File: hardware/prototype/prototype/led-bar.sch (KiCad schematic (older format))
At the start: 50 parts

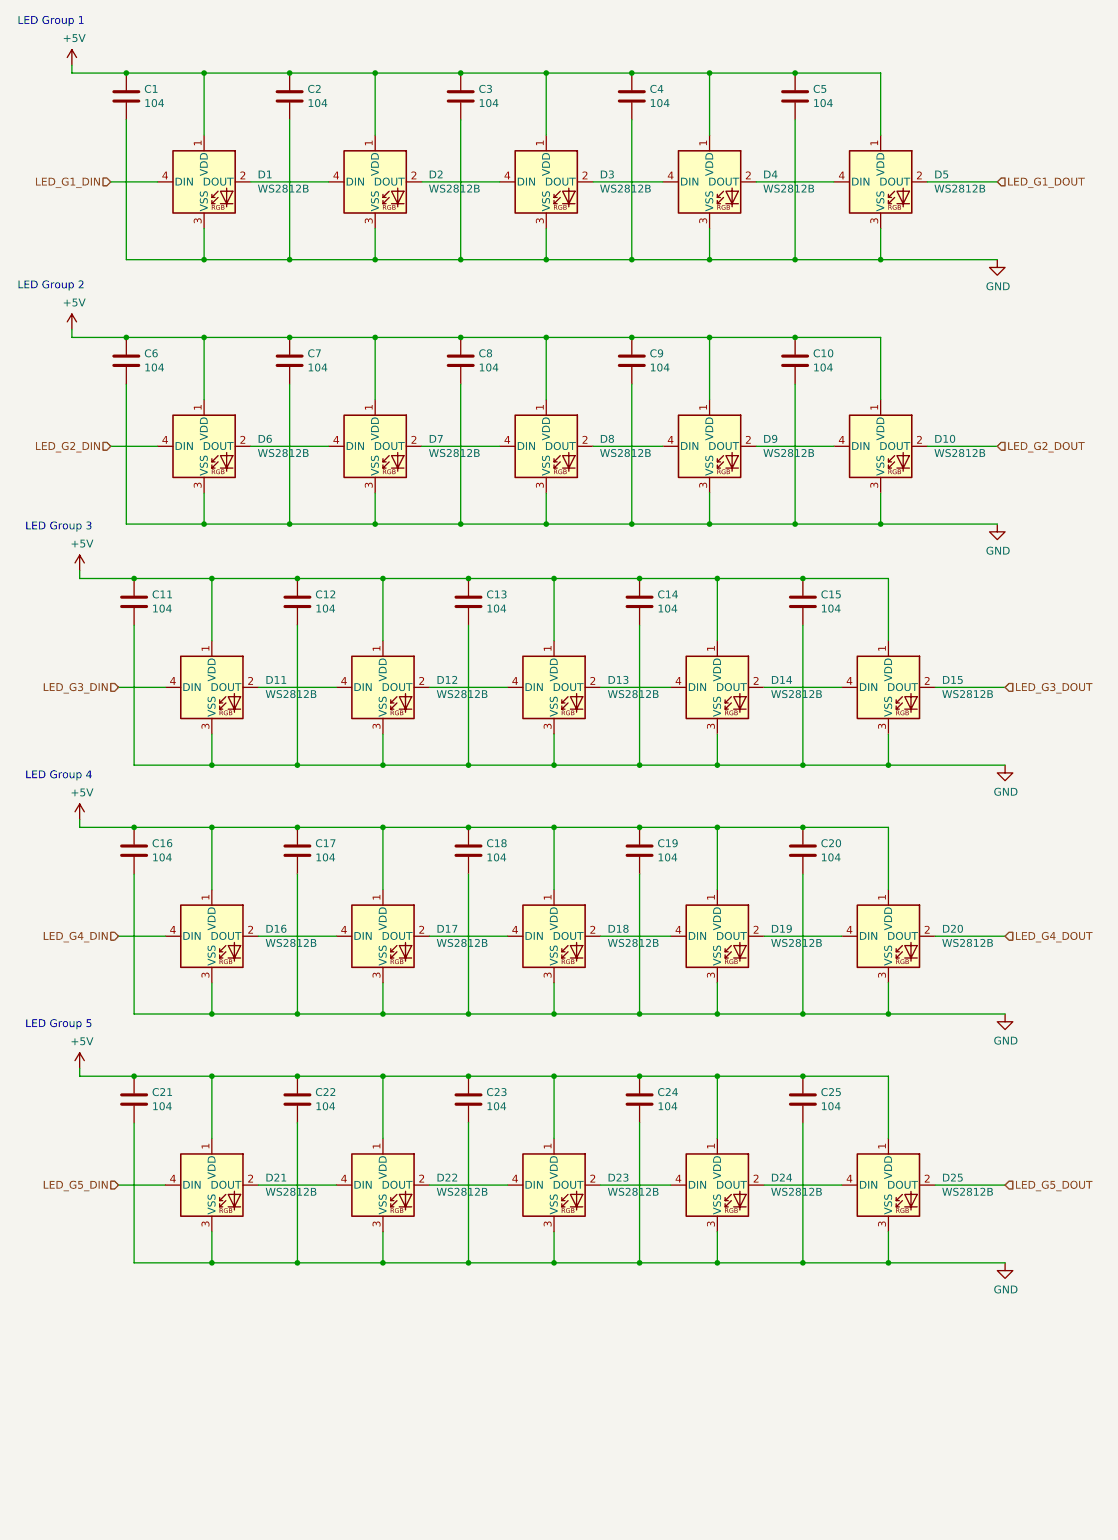
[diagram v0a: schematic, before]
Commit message: Update proto bar
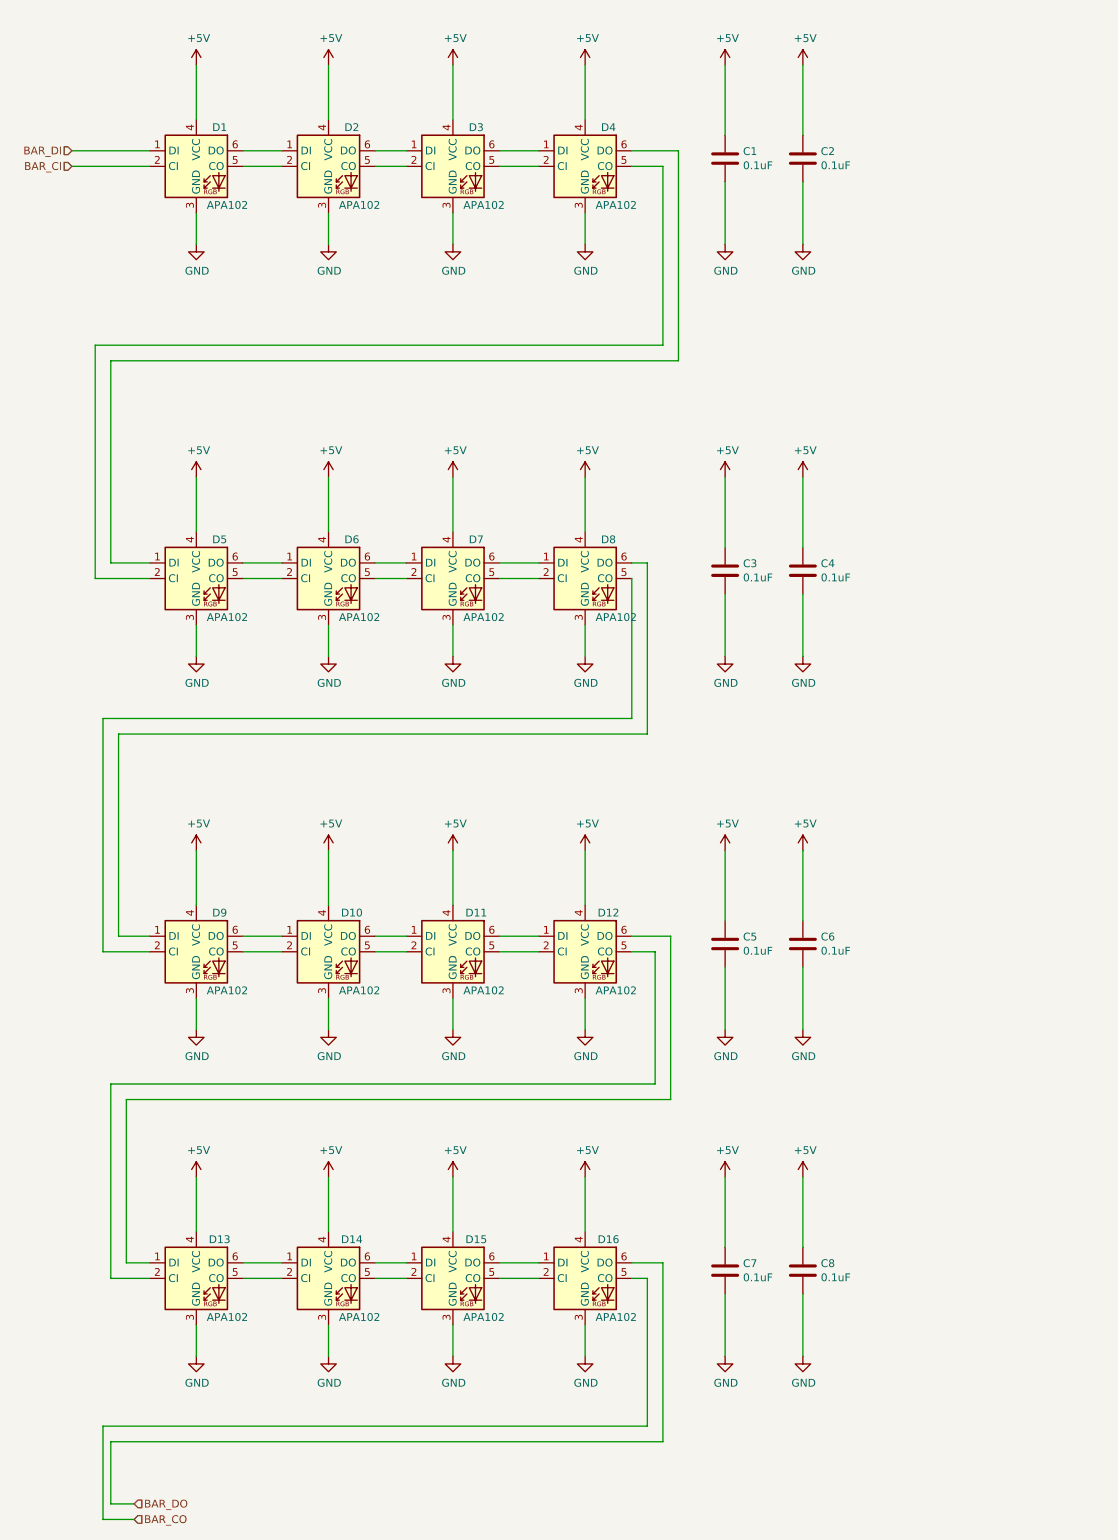
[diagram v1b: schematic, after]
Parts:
- removed C10, C11, C12, C13, C14, C15, C16, C17, C18, C19, C20, C21, C22, C23, C24, C25, C9: 104, Capacitor_SMD:C_0805_2012Metric, symbol Device:C
- removed D1, D10, D11, D12, D13, D14, D15, D16, D17, D18, D19, D2, D20, D21, D22, D23, D24, D25, D3, D4, D5, D6, D7, D8, D9: WS2812B, LED_SMD:LED_WS2812B_PLCC4_5.0x5.0mm_P3.2mm, symbol LED:WS2812B
- added D1, D10, D11, D12, D13, D14, D15, D16, D2, D3, D4, D5, D6, D7, D8, D9: APA102, LED_SMD:LED_RGB_5050-6, symbol LED:APA102
- C1, C2, C3, C4, C5, C6, C7, C8: value 104 -> 0.1uF; footprint Capacitor_SMD:C_0805_2012Metric -> Capacitor_SMD:C_0603_1608Metric
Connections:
- net +5V: now also D1.4 (VCC), D10.4 (VCC), D11.4 (VCC), D12.4 (VCC), D13.4 (VCC), D14.4 (VCC), D15.4 (VCC), D16.4 (VCC), D2.4 (VCC), D3.4 (VCC), D4.4 (VCC), D5.4 (VCC), D6.4 (VCC), D7.4 (VCC), D8.4 (VCC), D9.4 (VCC)
- net GND: now also D1.3 (GND), D10.3 (GND), D11.3 (GND), D12.3 (GND), D13.3 (GND), D14.3 (GND), D15.3 (GND), D16.3 (GND), D2.3 (GND), D3.3 (GND), D4.3 (GND), D5.3 (GND), D6.3 (GND), D7.3 (GND), D8.3 (GND), D9.3 (GND)
- new net: D1.5 (CO), D2.2 (CI)
- new net: D1.6 (DO), D2.1 (DI)
- new net: D2.5 (CO), D3.2 (CI)
- new net: D2.6 (DO), D3.1 (DI)
- new net: D3.5 (CO), D4.2 (CI)
- new net: D3.6 (DO), D4.1 (DI)
- new net: D4.5 (CO), D5.2 (CI)
- new net: D4.6 (DO), D5.1 (DI)
- new net: D5.5 (CO), D6.2 (CI)
- new net: D5.6 (DO), D6.1 (DI)
- new net: D6.5 (CO), D7.2 (CI)
- new net: D6.6 (DO), D7.1 (DI)
- new net: D7.5 (CO), D8.2 (CI)
- new net: D7.6 (DO), D8.1 (DI)
- new net: D8.5 (CO), D9.2 (CI)
- new net: D8.6 (DO), D9.1 (DI)
- new net: D10.2 (CI), D9.5 (CO)
- new net: D10.1 (DI), D9.6 (DO)
- new net: D10.5 (CO), D11.2 (CI)
- new net: D10.6 (DO), D11.1 (DI)
- new net: D11.5 (CO), D12.2 (CI)
- new net: D11.6 (DO), D12.1 (DI)
- new net: D12.5 (CO), D13.2 (CI)
- new net: D12.6 (DO), D13.1 (DI)
- new net: D13.5 (CO), D14.2 (CI)
- new net: D13.6 (DO), D14.1 (DI)
- new net: D14.5 (CO), D15.2 (CI)
- new net: D14.6 (DO), D15.1 (DI)
- new net: D15.5 (CO), D16.2 (CI)
- new net: D15.6 (DO), D16.1 (DI)
- new net BAR_CI: D1.2 (CI)
- new net BAR_CO: D16.5 (CO)
- new net BAR_DI: D1.1 (DI)
- new net BAR_DO: D16.6 (DO)
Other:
- note removed: "LED Group 1"
- note removed: "LED Group 2\n"
- note removed: "LED Group 3"
- note removed: "LED Group 4\n"
- note removed: "LED Group 5"
